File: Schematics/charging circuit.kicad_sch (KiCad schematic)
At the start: 21 parts, among them J1 amphenol pl00x and pl00y, J10 Amphenol PL00Y-301-10M8, J12 Amphenol PL00X-301-10M8, J16 Amphenol PL00X-301-10M8, J17 Amphenol PL00Y-301-10M8, J2 Conn_01x06, J3 Conn_01x08, SW2 SW_Push_Open

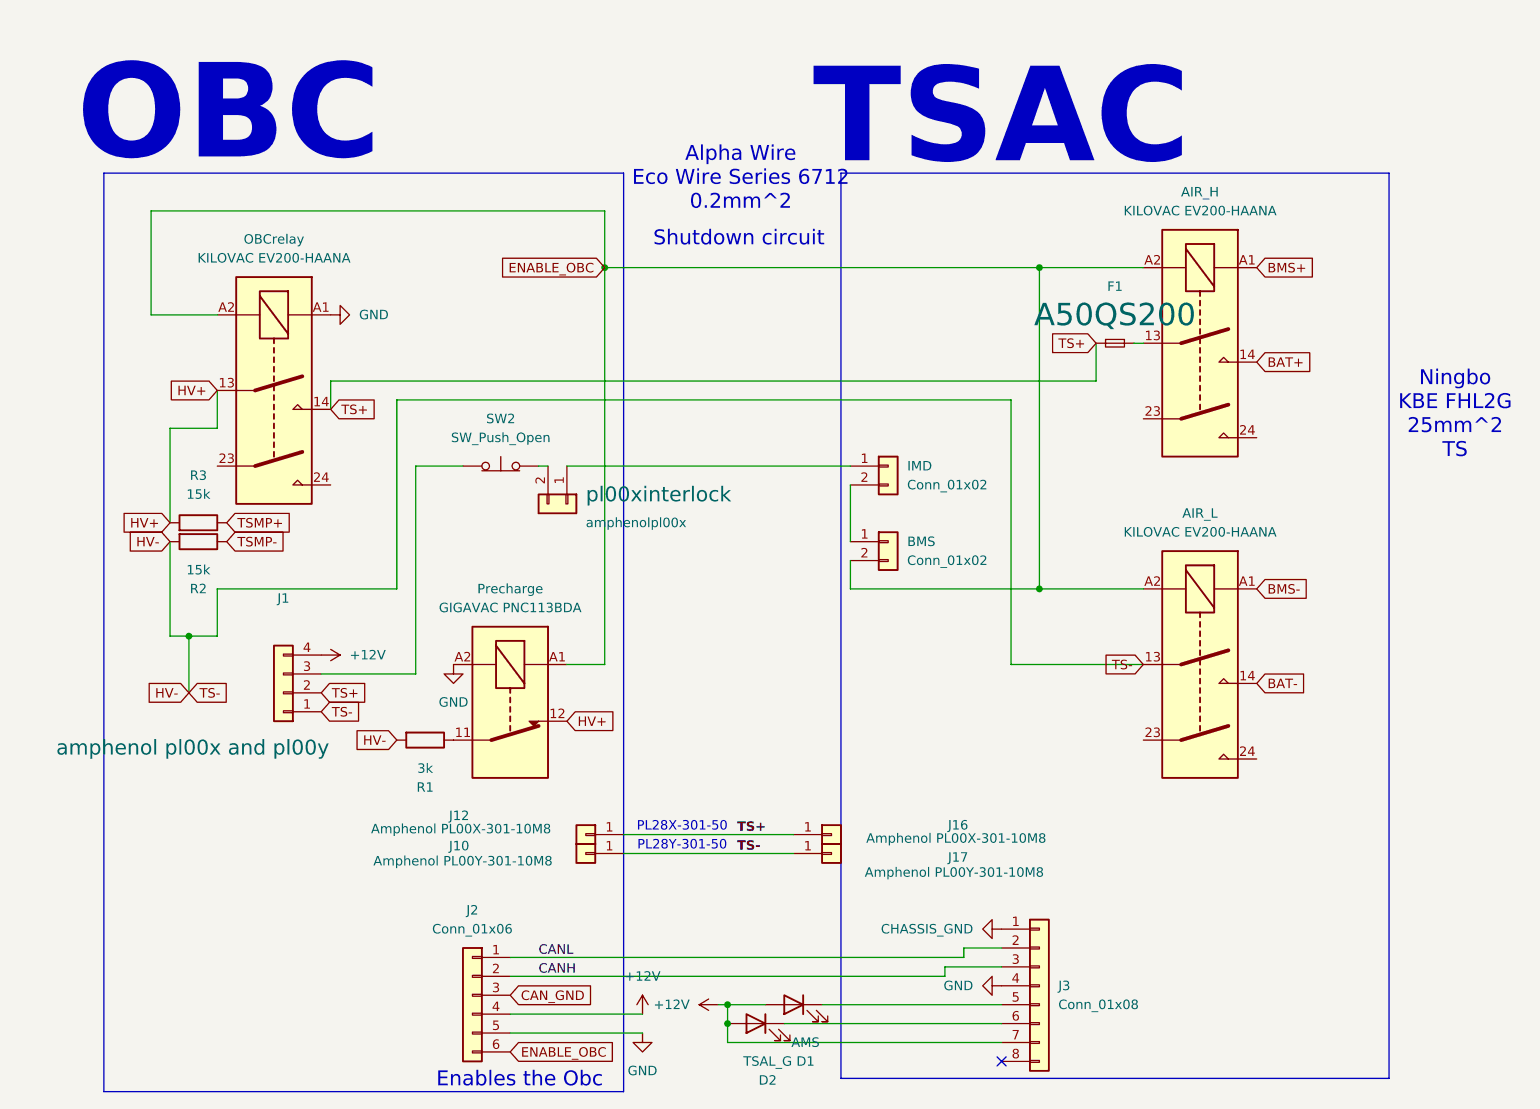
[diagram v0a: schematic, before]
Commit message: schematics push idk what are these idc
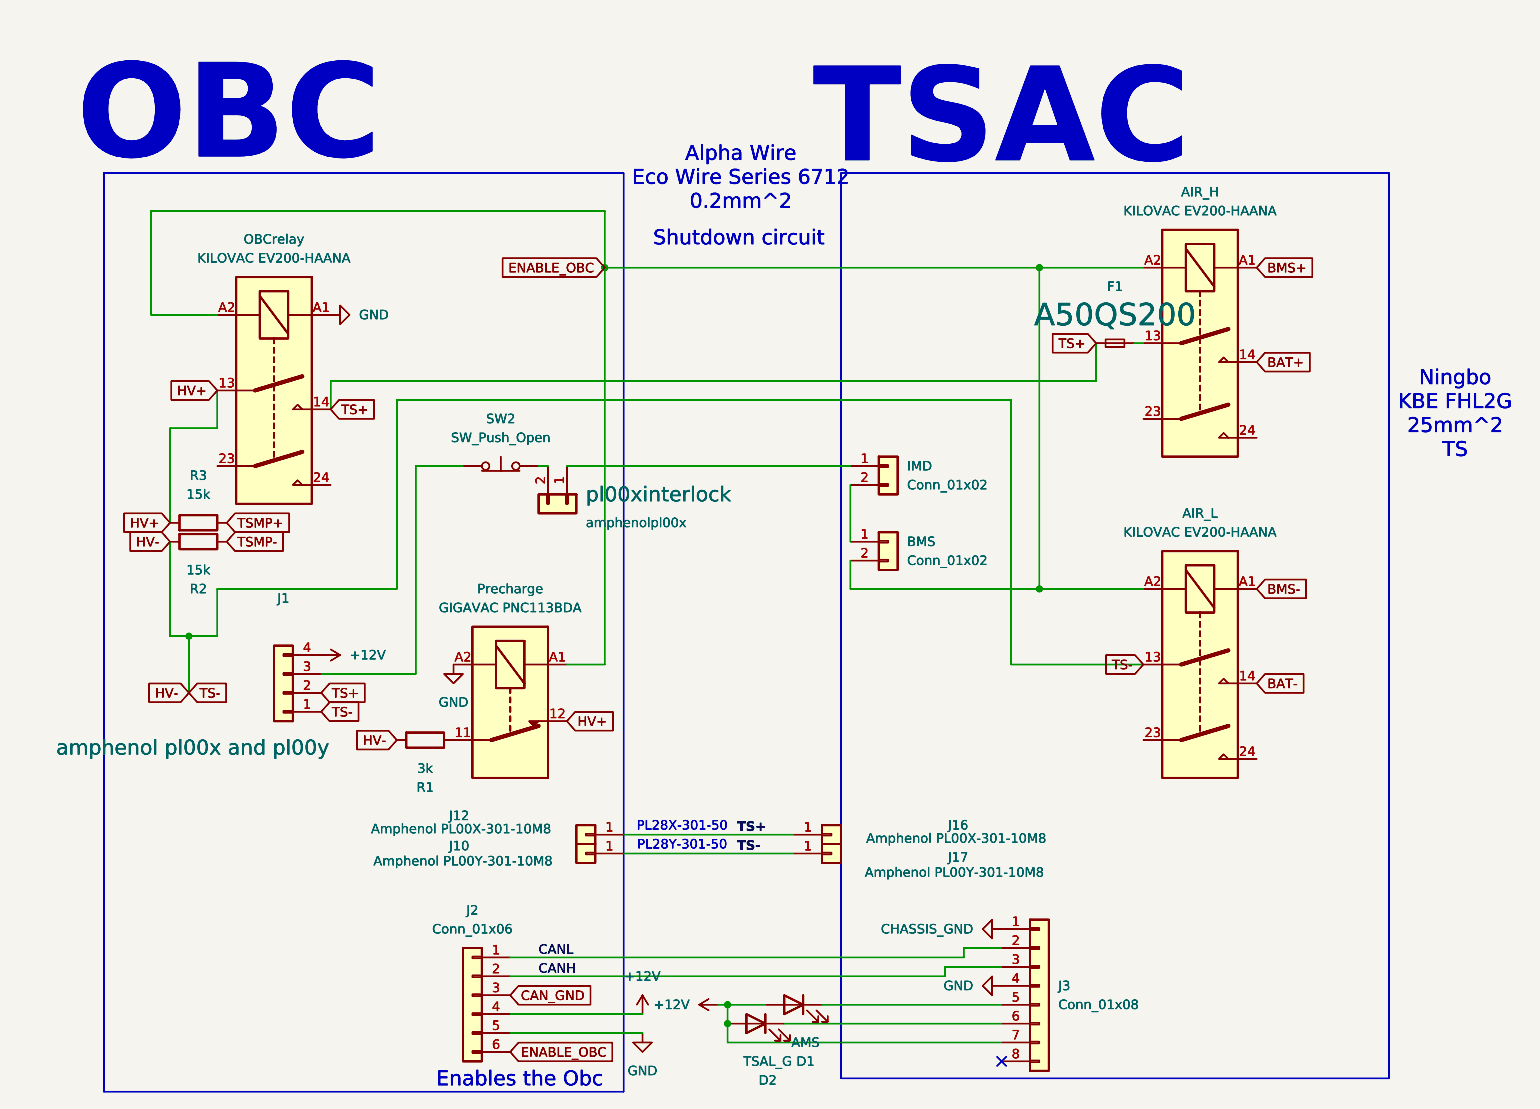
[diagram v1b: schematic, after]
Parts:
- added AIR_H, AIR_L, OBCrelay: KILOVAC EV200-HAANA, symbol Relay:Relay_DPST-NO
- added BMS, IMD: Conn_01x02, symbol Connector_Generic:Conn_01x02
- added D1: AMS, symbol Device:LED
- added D2: TSAL_G, symbol Device:LED
- added F1: A50QS200, symbol Device:Fuse_Small
- added J1: amphenol pl00x and pl00y, symbol Connector_Generic:Conn_01x04
- added J10, J17: Amphenol PL00Y-301-10M8, symbol Connector_Generic:Conn_01x01
- added J12, J16: Amphenol PL00X-301-10M8, symbol Connector_Generic:Conn_01x01
- added J2: Conn_01x06, symbol Connector_Generic:Conn_01x06
- added J3: Conn_01x08, symbol Connector_Generic:Conn_01x08
- added Precharge: GIGAVAC PNC113BDA, symbol Relay:Relay_SPST-NC
- added R1: 3k, symbol Device:R
- added R2, R3: 15k, symbol Device:R
- added SW2: SW_Push_Open, symbol Switch:SW_Push_Open
- added pl00xinterlock: amphenolpl00x, symbol Connector_Generic:Conn_01x02
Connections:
- net +12V: now also D1.2 (A), D2.2 (A), J1.4 (Pin_4), J2.4 (Pin_4), J3.7 (Pin_7)
- net BAT+: now also AIR_H.14
- net BAT-: now also AIR_L.14
- net BMS+: now also AIR_H.A1
- net BMS-: now also AIR_L.A1
- net CANH: now also J2.2 (Pin_2), J3.3 (Pin_3)
- net CANL: now also J2.1 (Pin_1), J3.2 (Pin_2)
- net CAN_GND: now also J2.3 (Pin_3)
- net CHASSIS_GND: now also J3.1 (Pin_1)
- net ENABLE_OBC: now also AIR_H.A2, AIR_L.A2, BMS.2 (Pin_2), J2.6 (Pin_6), OBCrelay.A2, Precharge.A1
- net GND: now also J2.5 (Pin_5), J3.4 (Pin_4), OBCrelay.A1, Precharge.A2
- net HV+: now also OBCrelay.13, Precharge.12, R3.2
- net HV-: now also AIR_L.13, J1.1 (Pin_1), J10.1 (Pin_1), J17.1 (Pin_1), R1.2, R2.2
- net TS+: now also F1.1, J1.2 (Pin_2), J12.1 (Pin_1), J16.1 (Pin_1), OBCrelay.14
- net TSMP+: now also R3.1
- net TSMP-: now also R2.1
- net at OBCrelay.23: now also OBCrelay.23
- net at OBCrelay.24: now also OBCrelay.24
- net at D1.1 (K), J3.5 (Pin_5): now also D1.1 (K), J3.5 (Pin_5)
- net at IMD.1 (Pin_1), pl00xinterlock.1 (Pin_1): now also IMD.1 (Pin_1), pl00xinterlock.1 (Pin_1)
- net at BMS.1 (Pin_1), IMD.2 (Pin_2): now also BMS.1 (Pin_1), IMD.2 (Pin_2)
- net at D2.1 (K), J3.6 (Pin_6): now also D2.1 (K), J3.6 (Pin_6)
- net at AIR_H.13, F1.2: now also AIR_H.13, F1.2
- net at AIR_H.23: now also AIR_H.23
- net at AIR_H.24: now also AIR_H.24
- net at Precharge.11, R1.1: now also Precharge.11, R1.1
- net at AIR_L.23: now also AIR_L.23
- net at AIR_L.24: now also AIR_L.24
- net at J3.8 (Pin_8): now also J3.8 (Pin_8)
- net at J1.3 (Pin_3), SW2.1 (A): now also J1.3 (Pin_3), SW2.1 (A)
- net at SW2.2 (B), pl00xinterlock.2 (Pin_2): now also SW2.2 (B), pl00xinterlock.2 (Pin_2)
- no-connect marks 1 -> 2
